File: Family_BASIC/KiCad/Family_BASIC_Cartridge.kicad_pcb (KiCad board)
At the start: 2 copper layers, 93 x 79.5 mm, 19 parts, among them IC1 Working RAM (62256), IC2 PRG ROM (27256), IC3 74HCT20, IC4 CHR ROM (27C64), SW1 BACKUP SW, SW2 RAM BANK SW

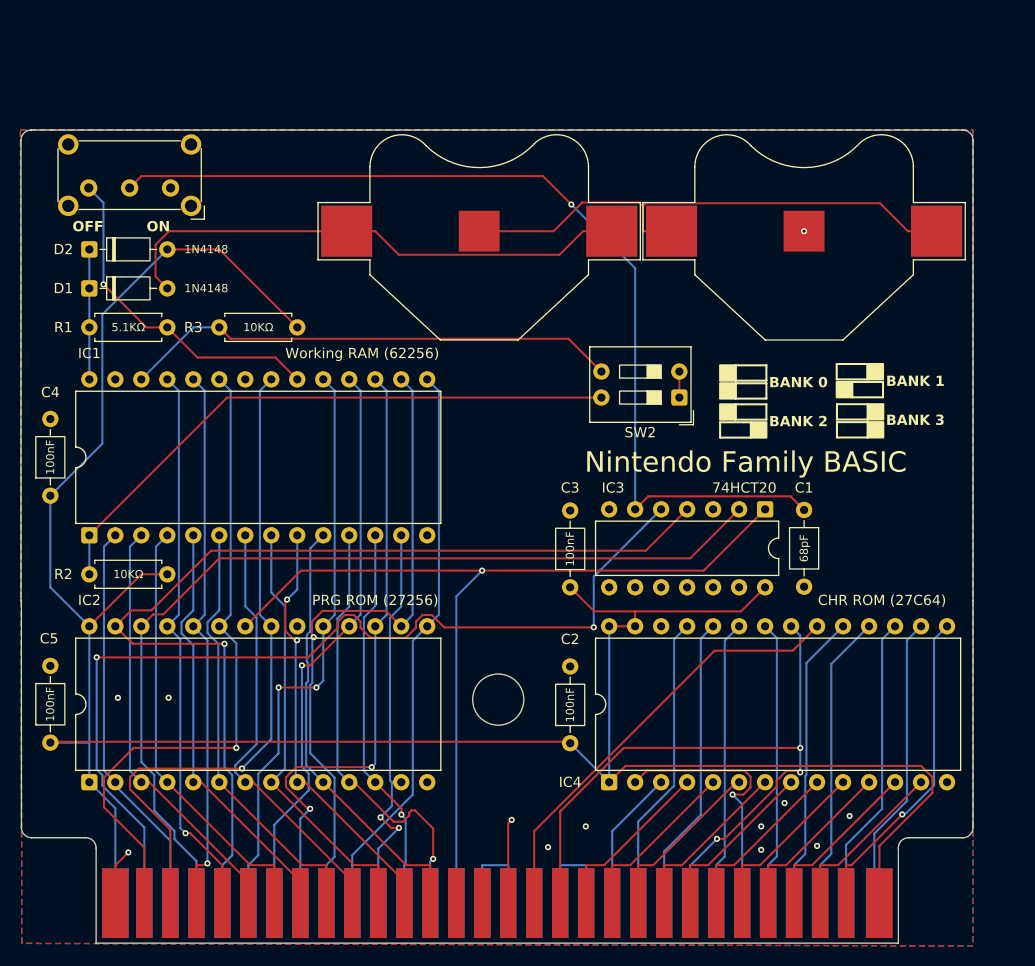
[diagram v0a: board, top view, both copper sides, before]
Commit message: Finalised initial Rev. A design
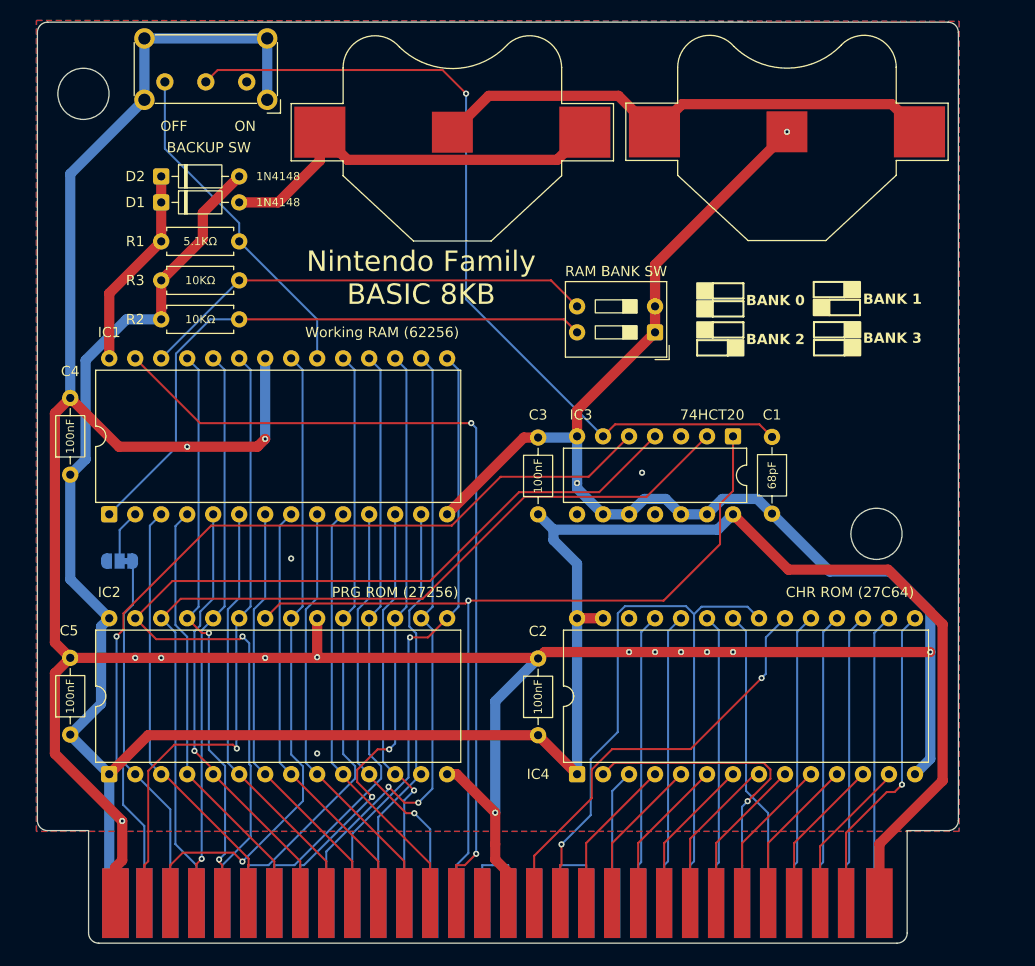
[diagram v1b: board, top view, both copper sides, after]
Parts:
- added JP1: A_{12} Enable, Jumper:SolderJumper-3_P1.3mm_Bridged12_RoundedPad1.0x1.5mm, B.Cu at (66.1, 110.1)
- moved R2 28.9 mm to (77.8, 86.5), turned to 180 degrees
- moved SW1 12.8 mm to (78.6, 63.3)
- moved D1 11.0 mm to (70.2, 75.1)
- moved R1 11.0 mm to (70.2, 78.9)
- moved BT1 10.0 mm to (98.7, 68.2)
- moved D2 10.0 mm to (70.2, 72.5)
- moved BT2 9.86 mm to (131.4, 68.2)
- moved C3 7.79 mm to (107.0, 105.6)
- moved IC3 7.79 mm to (126.1, 97.9)
- moved C1 7.79 mm to (129.9, 98.0)
- moved SW2 6.80 mm to (118.5, 87.8)
- moved R3 4.99 mm to (77.8, 82.7), turned to 180 degrees
- moved IC4 3.23 mm to (110.8, 131.0)
- moved C2 3.23 mm to (107.0, 127.1)
- moved C4 2.83 mm to (61.3, 101.7)
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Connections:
- net /SWA_{13} renamed /A_{13}SW
- net /SWA_{14} renamed /A_{14}SW
- H1 pad 14: /R/_{W} -> /R/~{W}
- IC1 pad 2: /A_{12} -> /A_{12}EN
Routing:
- net /GND: track 16.3 -> 377.9 mm, vias 12 -> 19
- net /R/~{W}: track 0.00 -> 83.9 mm, vias 0 -> 2
- net Net-(SW1-B): track 94.8 -> 83.4 mm
- net Net-(BT1-+): track 51.8 -> 40.5 mm
- net /V_{CC}: track 244.3 -> 236.1 mm
- net /O2: track 93.9 -> 86.3 mm, vias 2 -> 1
- net /RAMV_{CC}: track 12.7 -> 19.9 mm
- net /PA_{10}: track 68.3 -> 74.3 mm, vias 3 -> 1
- net /PA_{12}: track 26.1 -> 31.3 mm
- net /A_{12}EN: track 0.00 -> 5.20 mm
- net /A_{13}SW: track 48.9 -> 44.8 mm
- net /D_{6}: track 56.2 -> 60.1 mm, vias 1 -> 0
- net /D_{3}: track 55.2 -> 59.0 mm, vias 0 -> 1
- net /A_{11}: track 65.7 -> 62.1 mm
- net /A_{12}: track 39.1 -> 35.7 mm
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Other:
- board size 93 x 79.5 mm -> 90 x 90 mm
- board text added: "Nintendo Family BASIC 8KB"
- board text removed: "Nintendo Family BASIC"
